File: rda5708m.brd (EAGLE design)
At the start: 64.8 x 100 mm, 36 parts, among them IC1 RDA5807M, IC2 STM32L052K8U, Q1 32768Hz, U2 TPS73033, U3 MCP73831

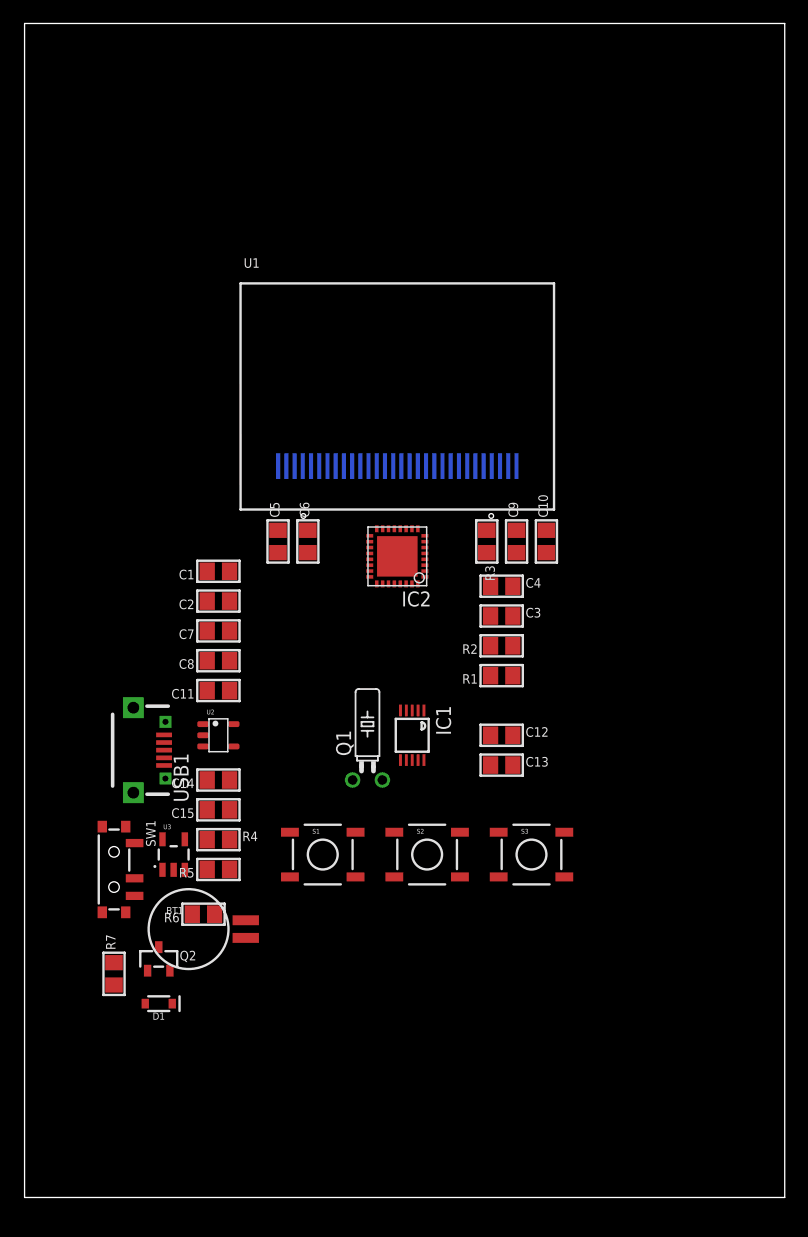
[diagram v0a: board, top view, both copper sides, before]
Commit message: fabricated version
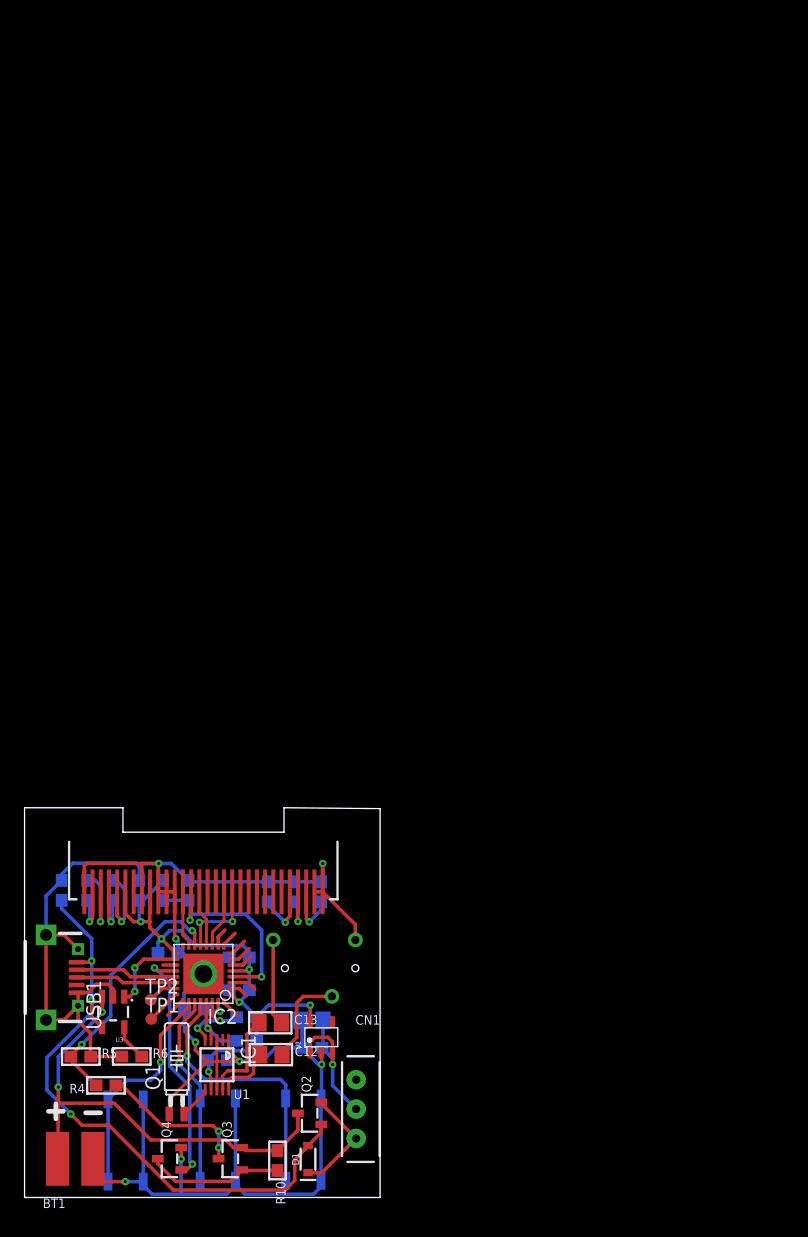
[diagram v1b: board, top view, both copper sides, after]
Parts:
- removed C8: 2.2uF, microbuilder:0805
- removed SW1: (no value), microbuilder:SPST_SMT_19192
- added CN1: (no value), rda5807m:AUDIO_3.5
- added Q3: IRLML5203, microbuilder:SOT23-R
- added Q4: (no value), microbuilder:SOT23-R
- added R10: 200k, microbuilder:0603
- added R8, R9: 10k, microbuilder:0603
- added S4: (no value), rda5807m:SWITCH-DPDT
- added TP1, TP2: TPTP10R, testpad:TP10R
- BT1: device SparkFun-Batteries:BATTCON-6.8MM -> rda5807m:JSTPH2
- C1, C10, C11, C15, C2, C3, C4, C5, C6, C7, C9, R1, R2, R3, R4, R5, R6, R7: device microbuilder:0805 -> microbuilder:0603
- Q1: device crystal:TC26H -> rda5807m:TC26H-SMD
- S1, S2, S3: device SparkFun-Retired:TACTILE-SWITCH-SMD -> rda5807m:TACTILE-SWITCH-SMD45
- U1: device microbuilder:UG-2864HSWEG01_0.96IN_WRAPAROUND -> rda5807m:OLED0.96
- U3: device SparkFun-IC-Power:SOT23-5 -> rda5807m:SOT23-5
- USB1: device con-hirose:MICRO_USB-B_4.85_HORN -> rda5807m:MICRO_USB-B_4.85_HORN
- moved U1 41.5 mm to (15.2, 25.4), turned to 180 degrees
- moved R2 40.1 mm to (18.9, 13.3), flipped to the bottom
- moved IC2 39.2 mm to (15.2, 19.1)
- moved R1 38.6 mm to (14.5, 16.0), flipped to the bottom
- moved C4 37.2 mm to (14.0, 26.2), flipped to the bottom, turned to 90 degrees
- moved C3 36.7 mm to (18.3, 20.4), flipped to the bottom
- moved C1 35.7 mm to (18.3, 17.7), flipped to the bottom, turned to 0 degrees
- moved C10 35.5 mm to (25.3, 26.0), flipped to the bottom, turned to 270 degrees
- moved C9 35.3 mm to (23.0, 26.0), flipped to the bottom, turned to 270 degrees
- moved R3 35.2 mm to (20.7, 26.0), flipped to the bottom, turned to 90 degrees
- moved C6 34.1 mm to (7.49, 26.2), flipped to the bottom, turned to 270 degrees
- moved C5 33.9 mm to (5.33, 26.2), flipped to the bottom, turned to 270 degrees
- moved C12 33.6 mm to (21.0, 12.2)
- moved Q1 32.8 mm to (13.0, 7.11)
- moved IC1 32.6 mm to (16.4, 11.3)
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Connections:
- net N$19 renamed SPI_DC
- net N$2 renamed VUSB
- net N$20 renamed SPI_SCK
- net N$21 renamed SPI_MOSI
- removed net 5.0V: C14.2, C15.2, R4.1, SW1.C, U2.1, U2.3
- new net +5V: C14.2, C15.2, S4.2, U2.1, U2.3
- new net N$18: Q3.1, Q4.3, R10.2
- new net N$19: IC2.9
- new net N$2: Q3.3, R4.1
- new net N$20: IC2.8
- new net N$21: IC2.7
- new net N$25: C13.2, CN1.3
- new net N$26: C12.2, CN1.2
- new net N$27: IC2.6
- new net N$29: IC2.16
- new net PA10: IC2.20, Q4.1
- new net PA8: IC2.18, U3.1
- new net PA9: IC2.19
- new net PC15: IC2.3
- new net SCLK: IC1.4, IC2.29, R2.1
- new net SDIO: IC1.5, IC2.30, R9.1
- new net SWCLK: IC2.24, TP1.TP
- new net SWDIO: IC2.23, TP2.TP
- new net VBAT: BT1.2, Q2.3, Q3.2, R10.1, U3.3
- net 3.3V: now also R2.2, R8.1, R9.2; no longer C8.2, R2.1
- net GND: now also BT1.1, CN1.1, Q1.P$1, Q4.2; no longer BT1.-, C8.1, Q1.1
- net N$1: now also Q1.P$2; no longer Q1.2
- net N$11: now also IC2.25; no longer IC1.4, IC2.29
- net N$15: now also S4.1; no longer SW1.B
- net N$16: now also IC2.10; no longer BT1.+, Q2.3, U3.3
- net N$4: now also IC2.32; no longer IC1.5, IC2.30
- net PC14: no longer U3.1
- net RST: now also R8.2; no longer R2.2
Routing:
- net GND: track 0.00 -> 183.8 mm, vias 0 -> 9
- net VUSB: track 0.00 -> 53.4 mm, vias 0 -> 3
- net 3.3V: track 0.00 -> 50.2 mm, vias 0 -> 6
- net VBAT: track 0.00 -> 39.6 mm, vias 0 -> 2
- net BTN3: track 0.00 -> 23.0 mm, vias 0 -> 1
- net PB0: track 0.00 -> 22.2 mm, vias 0 -> 2
- net PA10: track 0.00 -> 21.2 mm, vias 0 -> 2
- net RST: track 0.00 -> 19.5 mm, vias 0 -> 2
- net BTN1: track 0.00 -> 19.4 mm, vias 0 -> 1
- net BTN2: track 0.00 -> 16.5 mm, vias 0 -> 1
- net +5V: track 0.00 -> 13.8 mm, vias 0 -> 1
- net N$2: track 0.00 -> 12.7 mm, vias 0 -> 2
- net N$18: track 0.00 -> 11.7 mm
- net N$15: track 0.00 -> 9.63 mm
- net N$12: track 0.00 -> 8.72 mm
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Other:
- board size 64.8 x 100 mm -> 30.3 x 33.2 mm

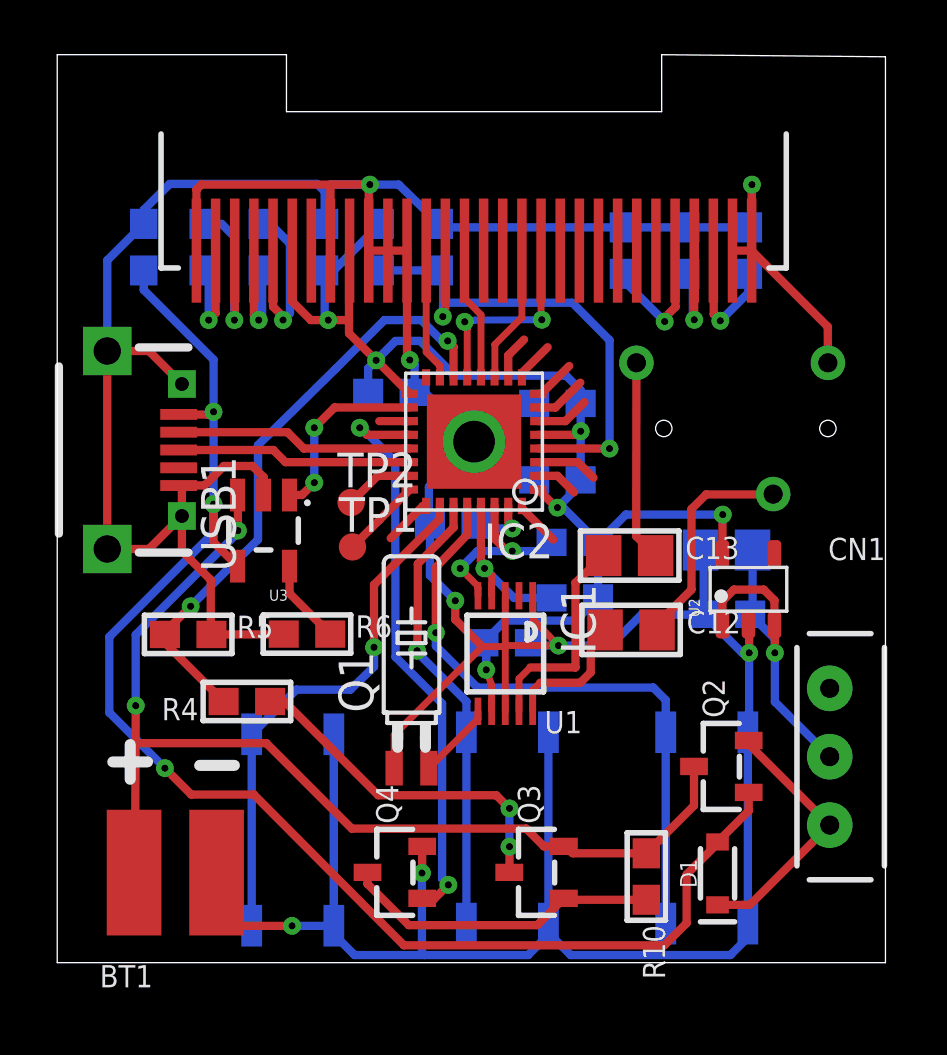
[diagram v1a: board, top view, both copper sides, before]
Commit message: fabricated release
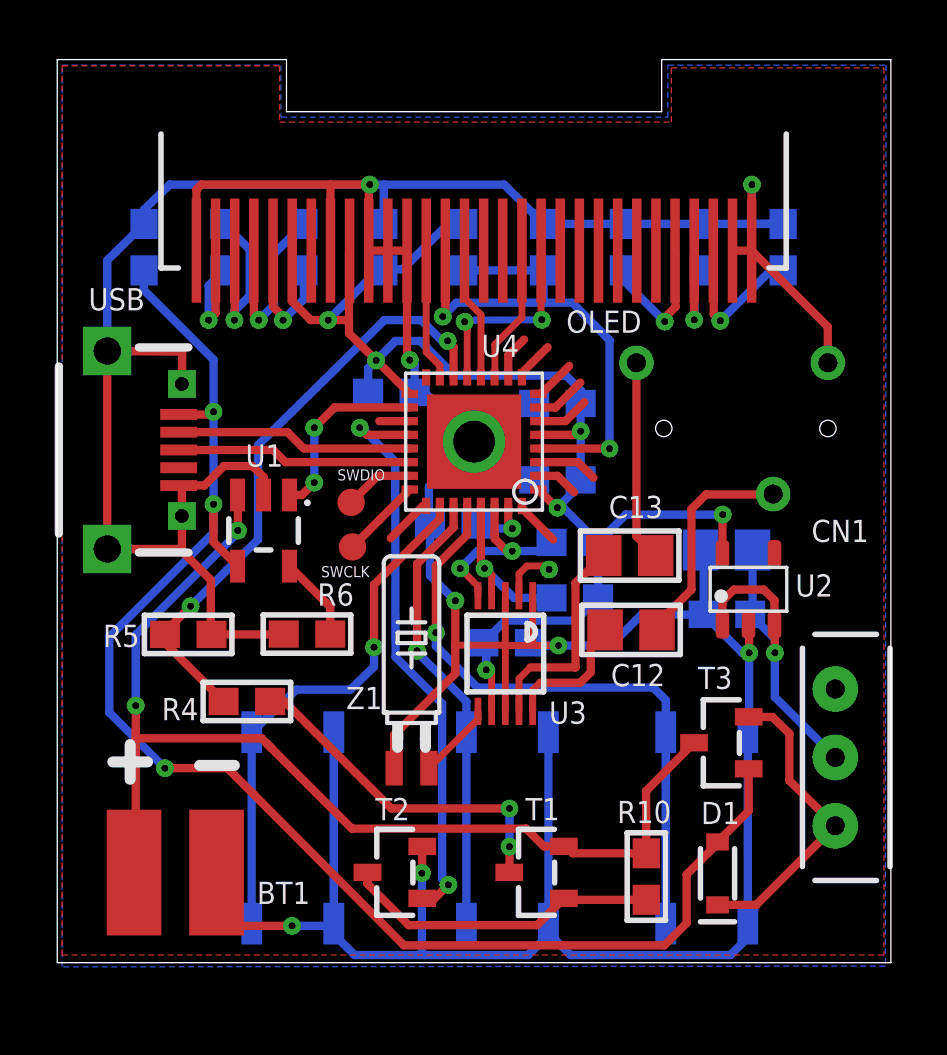
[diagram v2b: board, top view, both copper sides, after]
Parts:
- removed IC1: RDA5807M, rda5807m:MSOP10
- removed Q2: (no value), microbuilder:SOT23-R
- added OLED: (no value), rda5807m:OLED0.96
- added T3: (no value), microbuilder:SOT23-R
- U1: value (none) -> MCP73831; device rda5807m:OLED0.96 -> rda5807m:SOT23-5
- U3: value MCP73831 -> RDA5807M; device rda5807m:SOT23-5 -> rda5807m:MSOP10
- moved U1 12.3 mm to (7.54, 15.8)
- moved U3 9.92 mm to (16.4, 11.3)
- moved C4 3.81 mm to (17.8, 26.2)
- moved R8 3.05 mm to (14.9, 26.2)
- moved C7 2.16 mm to (11.9, 26.2)
- moved C6 1.52 mm to (9.02, 26.2), turned to 90 degrees
- moved C10 1.28 mm to (26.5, 26.2)
- moved C5 0.76 mm to (6.10, 26.2)
- moved C9 0.65 mm to (23.6, 26.2)
- moved S4 0.20 mm to (28.4, 7.51)
- moved R3 0.13 mm to (20.7, 26.2)
- moved S1 0.08 mm to (8.61, 4.93)
- renumbered IC2 to U4, Q1 to Z1, Q3 to T1, Q4 to T2, TP1 to SWCLK, TP2 to SWDIO, USB1 to USB
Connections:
- new net N$28: U3.2
- net 3.3V: now also OLED.6, OLED.9, U3.7; no longer IC1.7, U1.6, U1.9
- net GND: now also OLED.1, OLED.10, OLED.11, OLED.12, OLED.29, OLED.30, OLED.8, U1.2, U3.1, U3.3, U3.8; no longer IC1.1, IC1.3, IC1.8, U1.1, U1.10, U1.11, U1.12, U1.29, U1.30, U1.8, U3.2
- net N$1: now also U3.6; no longer IC1.6
- net N$10: now also U3.9; no longer IC1.9
- net N$14: now also U1.5; no longer U3.5
- net N$15: now also T3.2; no longer Q2.2
- net N$17: now also OLED.13; no longer U1.13
- net N$22: now also OLED.26; no longer U1.26
- net N$23: now also OLED.27; no longer U1.27
- net N$24: now also OLED.28; no longer U1.28
- net N$5: now also U3.10; no longer IC1.10
- net N$6: now also OLED.2; no longer U1.2
- net N$7: now also OLED.3; no longer U1.3
- net N$8: now also OLED.4; no longer U1.4
- net N$9: now also OLED.5; no longer U1.5
- net PA8: now also U1.1; no longer U3.1
- net RST: now also OLED.14; no longer U1.14
- net SCLK: now also U3.4; no longer IC1.4
- net SDIO: now also U3.5; no longer IC1.5
- net SPI_DC: now also OLED.15; no longer U1.15
- net SPI_MOSI: now also OLED.19; no longer U1.19
- net SPI_SCK: now also OLED.18; no longer U1.18
- net VBAT: now also T3.3, U1.3; no longer Q2.3, U3.3
- net VUSB: now also T3.1, U1.4; no longer Q2.1, U3.4
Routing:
- net GND: track 183.8 -> 187.0 mm
- net N$8: track 4.48 -> 6.81 mm
- net N$9: track 6.91 -> 4.82 mm
- net N$28: track 0.00 -> 2.07 mm, vias 0 -> 1
- net 3.3V: track 50.2 -> 52.0 mm
- net N$15: track 9.63 -> 11.3 mm
- net VBAT: track 39.6 -> 40.8 mm
- net SCLK: track 6.32 -> 7.49 mm
- net N$24: track 4.81 -> 5.77 mm
- net VUSB: track 53.4 -> 54.3 mm
- added copper zone on layer 1, net GND
- added copper zone on layer 16, net GND
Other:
- board size 30.3 x 33.2 mm -> 30.5 x 33 mm
